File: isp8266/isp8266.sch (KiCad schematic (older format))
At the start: 0 parts

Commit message: Complete power sch
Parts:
- added C? (x4): 10u, symbol Device:C_Small
- added C? (x6): 22u, symbol Device:C_Small
- added C? (x2): 1u, symbol Device:C_Small
- added D? (x2): LED_Small, symbol Device:LED_Small
- added L?: L_Small, symbol Device:L_Small
- added P?: USB_C_Plug, symbol Connector:USB_C_Plug
- added R? (x2): 5k1, symbol Device:R_Small
- added R?: 10k, symbol Device:R_Small
- added R?: 2, symbol Device:R_Small
- added R? (x2): 1k, symbol Device:R_Small
- added R?: 0.9, symbol Device:R_Small
- added SW?: SW_Push, symbol Switch:SW_Push
- added U?: ESP-12E, RF_Module:ESP-12E, symbol RF_Module:ESP-12E
- added U?: AP1117-33, Package_TO_SOT_SMD:SOT-223-3_TabPin2, symbol Regulator_Linear:AP1117-33
- added U?: IPS5306, symbol IPS5306:IPS5306
- added U?: CH340C, Package_SO:SOIC-16_3.9x9.9mm_P1.27mm, symbol Interface_USB:CH340C
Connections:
- new net: D?.2 (A), U?.2 (LED1)
- new net: R?.1, U?.3 (LED2), U?.4 (LED3)
- new net: SW?.1, U?.5 (KEY)
- new net: L?.1, U?.7 (SW)
- new net: P?.A5 (CC), R?.1
- new net: P?.B5 (VCONN), R?.1
- new net: R?.1, SW?.2
- new net: C?.1, R?.2
- new net: D?.1 (K), R?.1
- new net +3V3: C?.1, C?.1, D?.2 (A), U?.2 (VO)
- new net +5V: C?.1, C?.1, C?.1, C?.1, C?.1, C?.1, U?.3 (VI), U?.8 (VOUT)
- new net BAT: C?.1, L?.2, R?.1
- new net D+: P?.A6 (D+)
- new net D-: P?.A7 (D-)
- new net GND: C?.2, C?.2, C?.2, C?.2, C?.2, C?.2, C?.2, C?.2, C?.2, C?.2, C?.2, C?.2, D?.1 (K), P?.A1 (GND), P?.A10 (RX2-), P?.A11 (RX2+), P?.A12 (GND), P?.A2 (TX1+), P?.A3 (TX1-), P?.B1 (GND), P?.B10 (RX1-), P?.B11 (RX1+), P?.B12 (GND), P?.B2 (TX2+), P?.B3 (TX2-), P?.S1 (SHIELD), R?.2, R?.2, R?.2, R?.2, U?.1 (GND), U?.9 (GND)
- new net IC_BAT: C?.1, R?.2, R?.2, U?.6 (BAT)
- new net VBUS: C?.1, P?.A4 (VBUS), P?.A9 (VBUS), P?.B4 (VBUS), P?.B9 (VBUS), R?.1, U?.1 (VIN)
- no-connect marks 0 -> 2

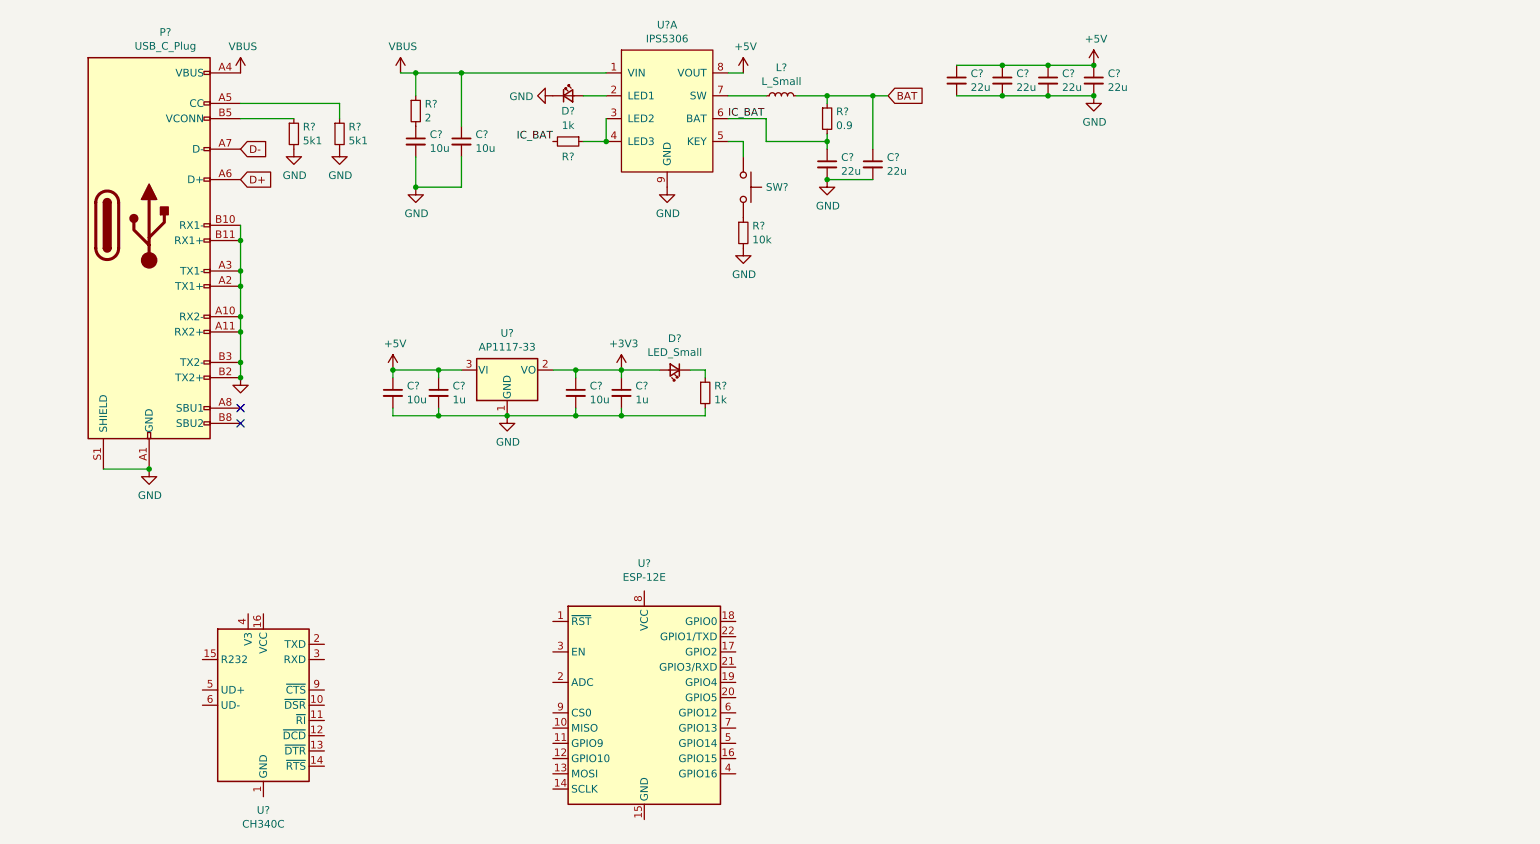
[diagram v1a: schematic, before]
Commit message: Complete all peripherals
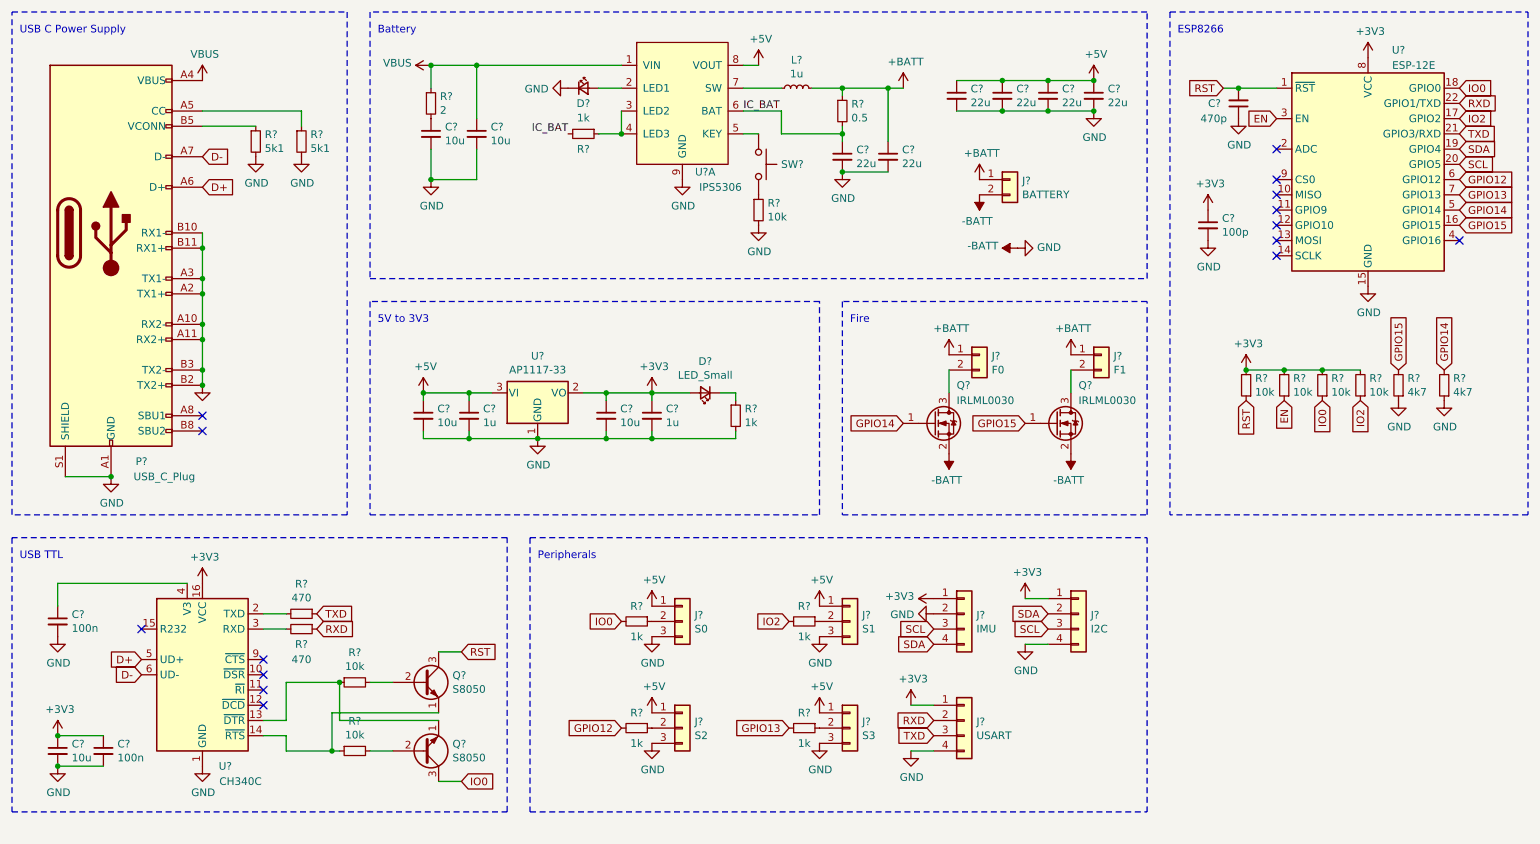
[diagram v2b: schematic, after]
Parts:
- added C? (x2): 100n, symbol Device:C_Small
- added C?: 10u, symbol Device:C_Small
- added C?: 470p, symbol Device:C_Small
- added C?: 100p, symbol Device:C_Small
- added J?: S0, symbol Connector_Generic:Conn_01x03
- added J?: S1, symbol Connector_Generic:Conn_01x03
- added J?: S2, symbol Connector_Generic:Conn_01x03
- added J?: S3, symbol Connector_Generic:Conn_01x03
- added J?: IMU, symbol Connector_Generic:Conn_01x04
- added J?: USART, symbol Connector_Generic:Conn_01x04
- added J?: F0, symbol Connector_Generic:Conn_01x02
- added J?: F1, symbol Connector_Generic:Conn_01x02
- added J?: BATTERY, symbol Connector_Generic:Conn_01x02
- added J?: I2C, symbol Connector_Generic:Conn_01x04
- added Q? (x2): S8050, Package_TO_SOT_THT:TO-92_Inline, symbol Transistor_BJT:S8050
- added Q? (x2): IRLML0030, Package_TO_SOT_SMD:SOT-23, symbol Transistor_FET:IRLML0030
- added R? (x2): 470, symbol Device:R_Small
- added R? (x6): 10k, symbol Device:R_Small
- added R? (x2): 4k7, symbol Device:R_Small
- added R? (x4): 1k, symbol Device:R_Small
- L?: value L_Small -> 1u
- R?: value 0.9 -> 0.5
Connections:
- net GND is gone; now on net -BATT: C?.2, C?.2, C?.2, C?.2, C?.2, C?.2, C?.2, C?.2, C?.2, C?.2, C?.2, C?.2, D?.1 (K), P?.A1 (GND), P?.A10 (RX2-), P?.A11 (RX2+), P?.A12 (GND), P?.A2 (TX1+), P?.A3 (TX1-), P?.B1 (GND), P?.B10 (RX1-), P?.B11 (RX1+), P?.B12 (GND), P?.B2 (TX2+), P?.B3 (TX2-), P?.S1 (SHIELD), R?.2, R?.2, R?.2, R?.2, U?.1 (GND), U?.9 (GND)
- net +3V3: now also U?.16 (VCC), U?.8 (VCC), C?.1, C?.1, C?.1, J?.1 (Pin_1), J?.1 (Pin_1), J?.1 (Pin_1), R?.2, R?.2, R?.2, R?.2
- net +5V: now also J?.1 (Pin_1), J?.1 (Pin_1), J?.1 (Pin_1), J?.1 (Pin_1)
- net D+: now also U?.5 (UD+)
- net D-: now also U?.6 (UD-)
- net RST: now reaches U?.1 (~RST)
- net RST: now also C?.2, Q?.3 (C), R?.1
- net -BATT: now reaches U?.15 (GND)
- net -BATT: now also U?.1 (GND), C?.1, C?.2, C?.2, C?.2, C?.2, J?.2 (Pin_2), J?.2 (Pin_2), J?.3 (Pin_3), J?.3 (Pin_3), J?.3 (Pin_3), J?.3 (Pin_3), J?.4 (Pin_4), J?.4 (Pin_4), Q?.2 (S), Q?.2 (S), R?.1, R?.1
- net GPIO15: now reaches U?.16 (GPIO15)
- net GPIO15: now also Q?.1 (G), R?.2
- net IO2: now reaches U?.17 (GPIO2)
- net IO2: now also R?.1, R?.2
- net IO0: now reaches U?.18 (GPIO0)
- net IO0: now also Q?.3 (C), R?.1, R?.2
- net SDA: now reaches U?.19 (GPIO4)
- net SDA: now also J?.2 (Pin_2), J?.4 (Pin_4)
- net SCL: now reaches U?.20 (GPIO5)
- net SCL: now also J?.3 (Pin_3), J?.3 (Pin_3)
- net TXD: now reaches U?.21 (GPIO3/RXD)
- net TXD: now also J?.3 (Pin_3), R?.1
- net RXD: now reaches U?.22 (GPIO1/TXD)
- net RXD: now also J?.2 (Pin_2), R?.1
- net EN: now reaches U?.3 (EN)
- net EN: now also R?.1
- net GPIO14: now reaches U?.5 (GPIO14)
- net GPIO14: now also Q?.1 (G), R?.2
- net GPIO12: now reaches U?.6 (GPIO12)
- net GPIO12: now also R?.2
- net GPIO13: now reaches U?.7 (GPIO13)
- net GPIO13: now also R?.2
- net at U?.13 (~DTR): now also Q?.1 (E), R?.1
- net at U?.14 (~RTS): now also Q?.1 (E), R?.1
- net at U?.2 (TXD): now also R?.2
- net at U?.3 (RXD): now also R?.2
- net at U?.4 (V3): now also C?.1
- net BAT renamed +BATT
- net +BATT: now also J?.1 (Pin_1), J?.1 (Pin_1), J?.1 (Pin_1)
- new net: Q?.2 (B), R?.2 (x2)
- new net: J?.2 (Pin_2), R?.1 (x4)
- new net: J?.2 (Pin_2), Q?.3 (D) (x2)
- no-connect marks 2 -> 15
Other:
- note added: "5V to 3V3"
- note added: "Battery"
- note added: "ESP8266"
- note added: "Fire"
- note added: "Peripherals"
- note added: "USB C Power Supply"
- note added: "USB TTL"
- moved on the sheet: C?, D?, L?, P?, R?, SW?, U?, U?A
